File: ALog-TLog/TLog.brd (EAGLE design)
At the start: 124.1 x 45.3 mm, 111 parts, among them IC1 ATMEGA644M, J6 5.5x2.1mm Barrel, Q11 MOSFET-NCH-BSS138, Q12 MOSFET_PCH-IRLML2244, Q5 MOSFET_PCH-IRLML2244, Q6 MOSFET_PCH-IRLML2244, Q7 MOSFET_PCH-IRLML2244, Q8 MOSFET-NCH-BSS138, Q9 MOSFET-NCH-BSS138, U2 FT231X-Q, U3 915MHz, U4 SX1509, X2 87832-14

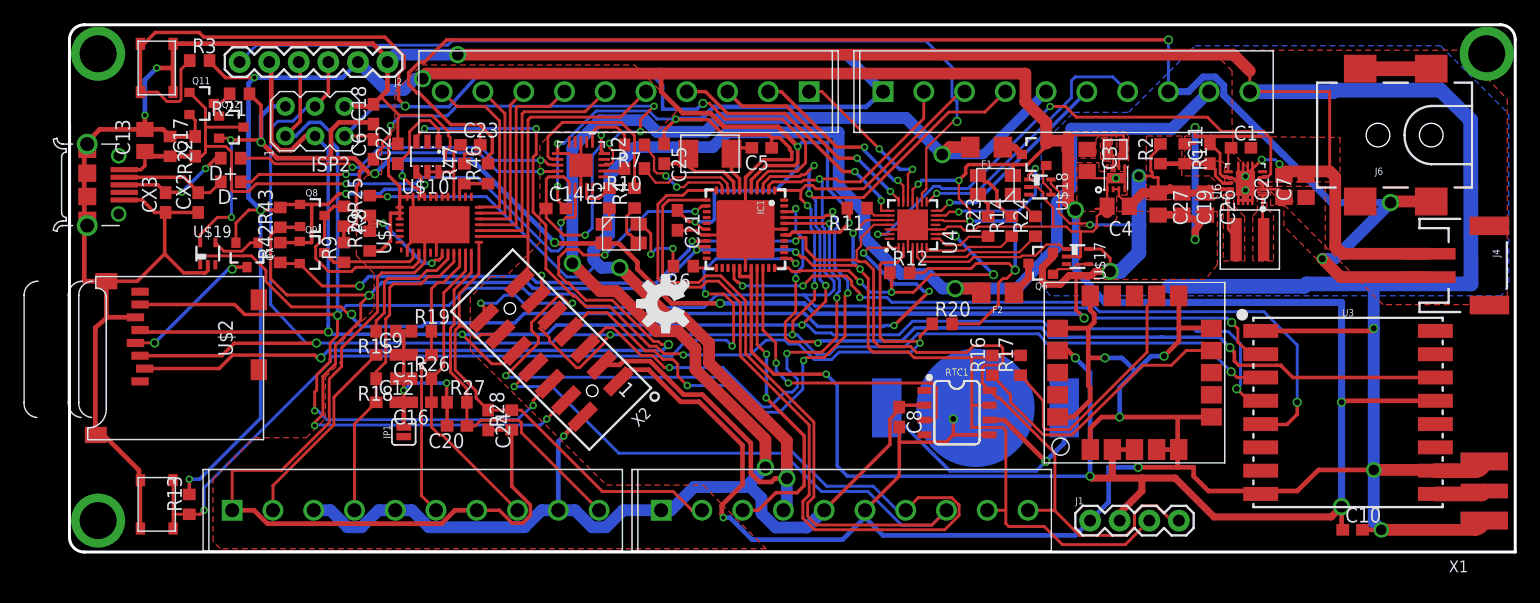
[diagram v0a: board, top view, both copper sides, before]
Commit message: Updated Gerbers, ready for final review
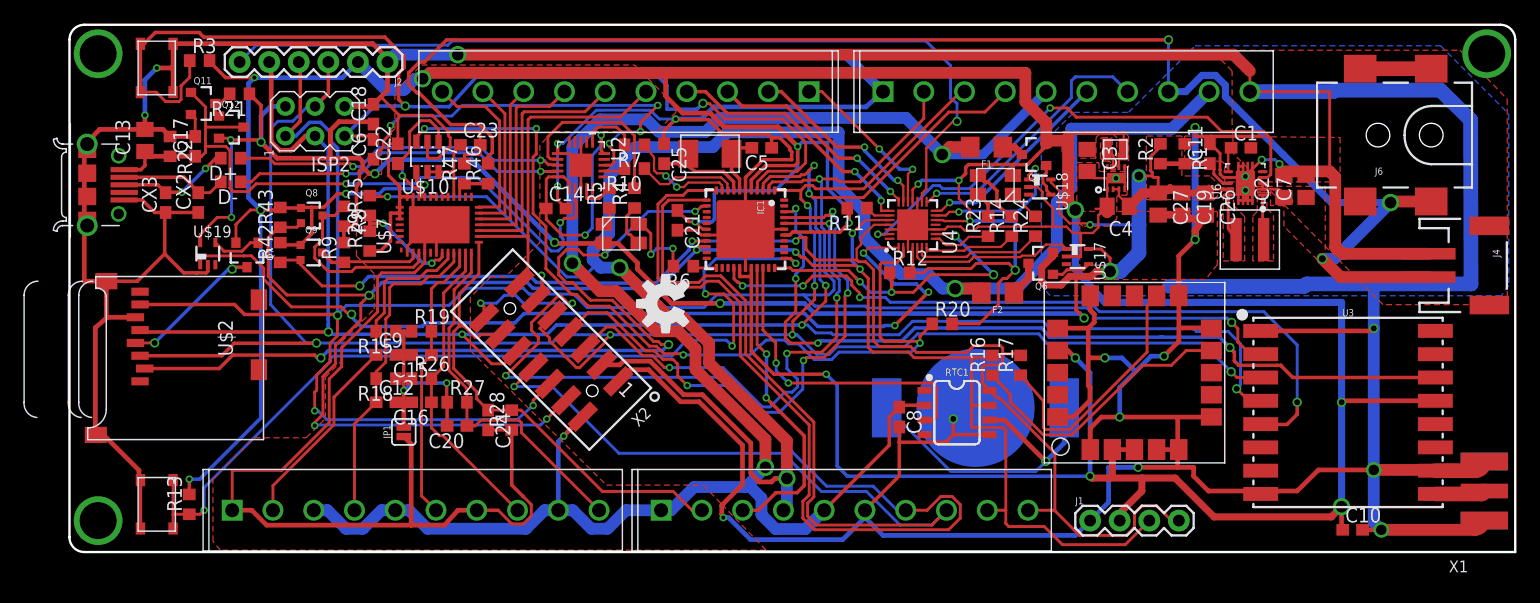
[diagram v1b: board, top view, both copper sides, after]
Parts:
- Q8, Q9: value MOSFET-NCH-BSS138 -> 310mA/60V/1.6Ω; device bschulz:SOT23-3 -> bschulz:SOT323
- moved Q11 0.13 mm to (11.6, 38.6)
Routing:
- net GND: track 818.7 -> 834.6 mm
- net DTR: track 35.2 -> 35.8 mm
- net EXT_3.3V: track 161.3 -> 161.9 mm
